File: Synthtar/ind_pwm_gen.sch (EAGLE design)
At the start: 23 parts, among them IC1 74HC164N, IC2 4081N, IC3 555

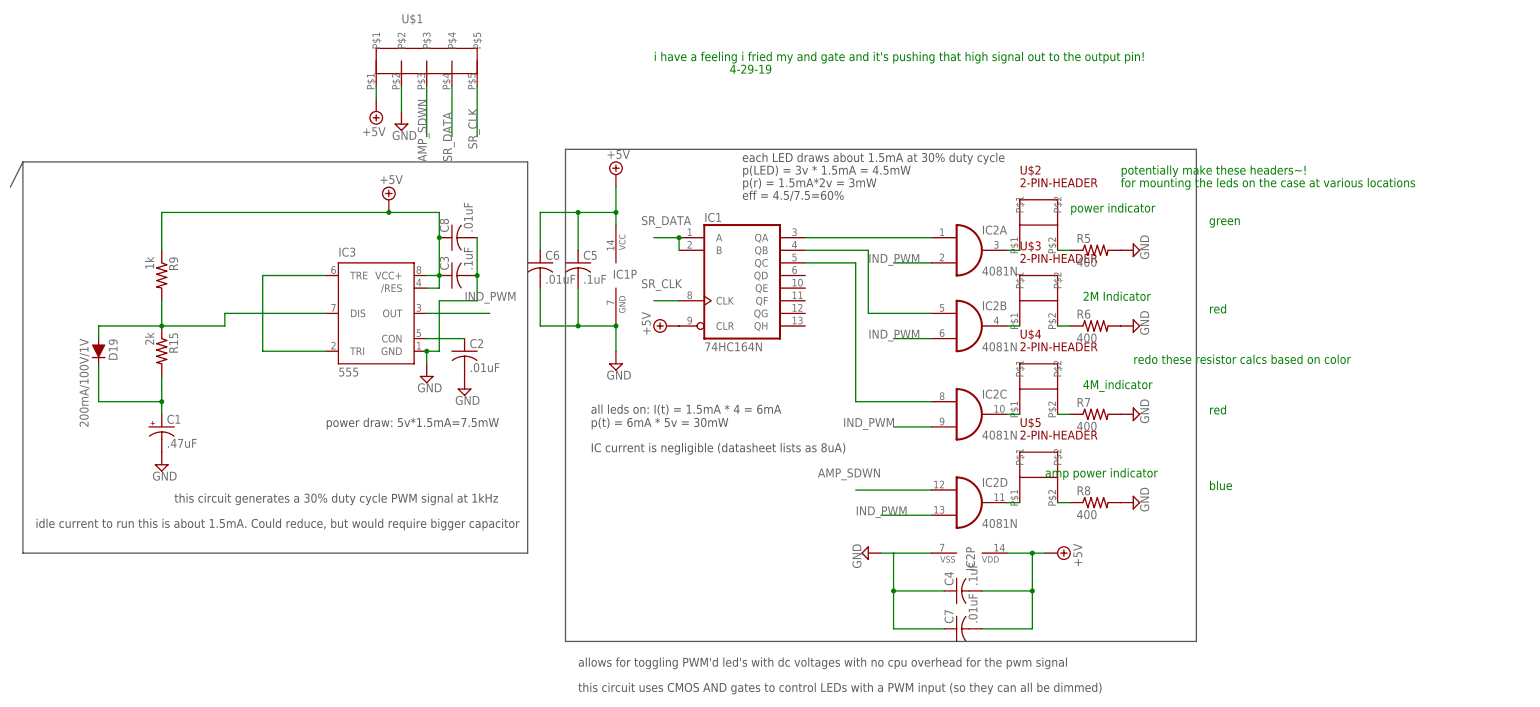
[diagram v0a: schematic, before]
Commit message: making boards and taking care of business
honestly haven't made a commit in so fucking long
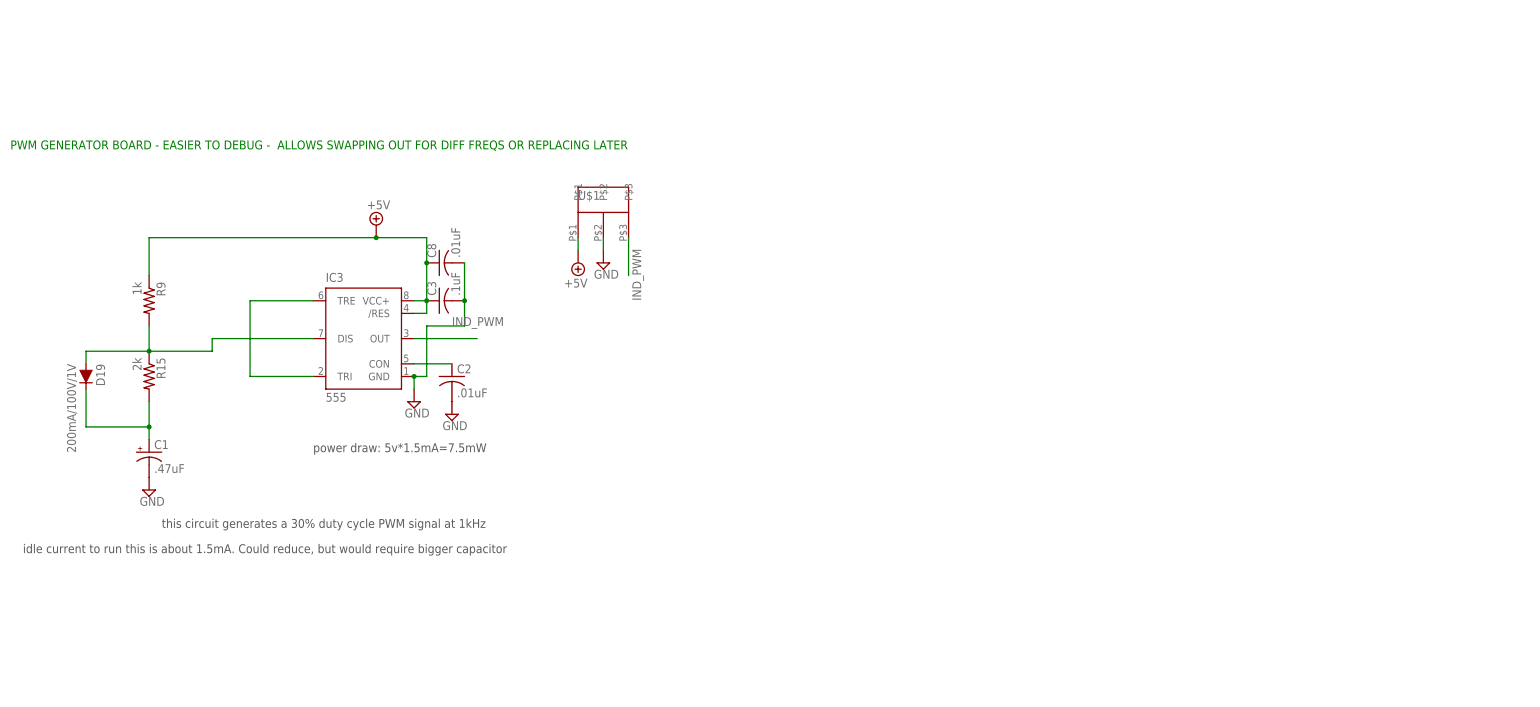
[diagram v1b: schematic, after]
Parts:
- removed C4, C5: .1uF, rcl:C-US025-030X050
- removed C6, C7: .01uF, rcl:C-US025-030X050
- removed IC1: 74HC164N, 74xx-us:74HC164N
- removed IC2: 4081N, 40xx:4081N
- removed R5, R6, R7, R8: 400, rcl:R-US_0204/7
- removed U$2, U$3, U$4, U$5: 2-PIN-HEADER, mask_lbr:2-PIN-HEADER
- U$1: value 5-PIN-HEADER -> 3-PIN-HEADER; device mask_lbr:5-PIN-HEADER -> mask_lbr:3-PIN-HEADER
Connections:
- removed net AMP_SDWN: IC2D.I0, U$1.P$3
- removed net N$14: IC1A.QA, IC2A.I0
- removed net N$17: IC1A.QB, IC2B.I0
- removed net N$47: IC2A.O, U$2.P$1
- removed net N$49: IC1A.QC, IC2C.I0
- removed net N$50: R5.1, U$2.P$2
- removed net N$51: IC2B.O, U$3.P$1
- removed net N$54: R6.1, U$3.P$2
- removed net N$55: IC2C.O, U$4.P$1
- removed net N$56: R7.1, U$4.P$2
- removed net N$57: IC2D.O, U$5.P$1
- removed net N$58: R8.1, U$5.P$2
- removed net SR_CLK: IC1A.CLK, U$1.P$5
- removed net SR_DATA: IC1A.A, IC1A.B, U$1.P$4
- net +5V: no longer C4.2, C5.1, C6.1, C7.2, IC1A.CLR, IC1P.VCC, IC2P.VDD
- net GND: no longer C4.1, C5.2, C6.2, C7.1, IC1P.GND, IC2P.VSS, R5.2, R6.2, R7.2, R8.2
- net IND_PWM: now also U$1.P$3; no longer IC2A.I1, IC2B.I1, IC2C.I1, IC2D.I1
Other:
- note added: "PWM GENERATOR BOARD - EASIER TO DEBUG - ALLOWS SWAPPING OUT FOR DIFF FREQS OR REPLACING LATER"
- note removed: "2M Indicator"
- note removed: "4-29-19"
- note removed: "4M_indicator"
- note removed: "IC current is negligible (datasheet lists as 8uA)"
- note removed: "all leds on: I(t) = 1.5mA * 4 = 6mA p(t) = 6mA * 5v = 30mW"
- note removed: "allows for toggling PWM'd led's with dc voltages with no cpu overhead for the pwm signal"
- note removed: "amp power indicator"
- note removed: "blue"
- note removed: "each LED draws about 1.5mA at 30% duty cycle"
- note removed: "eff = 4.5/7.5=60%"
- note removed: "for mounting the leds on the case at various locations"
- note removed: "green"
- note removed: "i have a feeling i fried my and gate and it's pushing that high signal out to the output pin!"
- note removed: "p(LED) = 3v * 1.5mA = 4.5mW"
- note removed: "p(r) = 1.5mA*2v = 3mW"
- note removed: "potentially make these headers~!"
- note removed: "power indicator"
- note removed: "red"
- note removed: "redo these resistor calcs based on color"
- note removed: "this circuit uses CMOS AND gates to control LEDs with a PWM input (so they can all be dimmed)"
- moved on the sheet: C1, C2, C3, C8, D19, IC3, R15, R9
